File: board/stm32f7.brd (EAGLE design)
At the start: 38 x 37.7 mm, 34 parts, among them Q1 8MHz, U1 STM32F722XX, X1 MINI-USB-32005-201

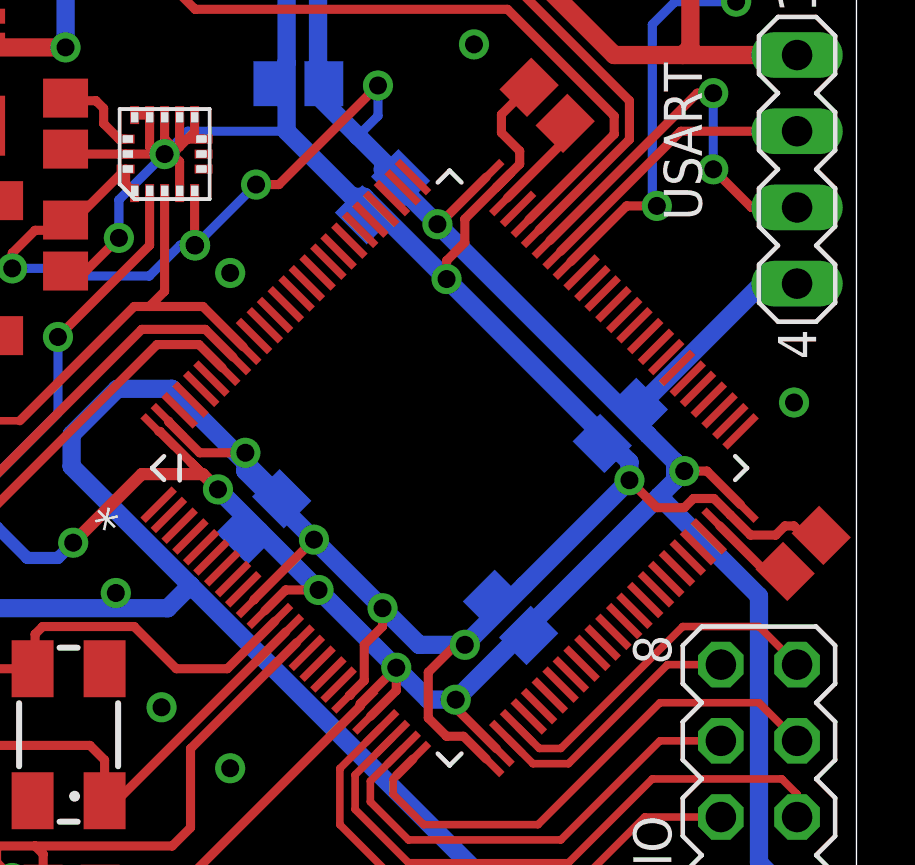
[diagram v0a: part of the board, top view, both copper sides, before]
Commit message: ir cam
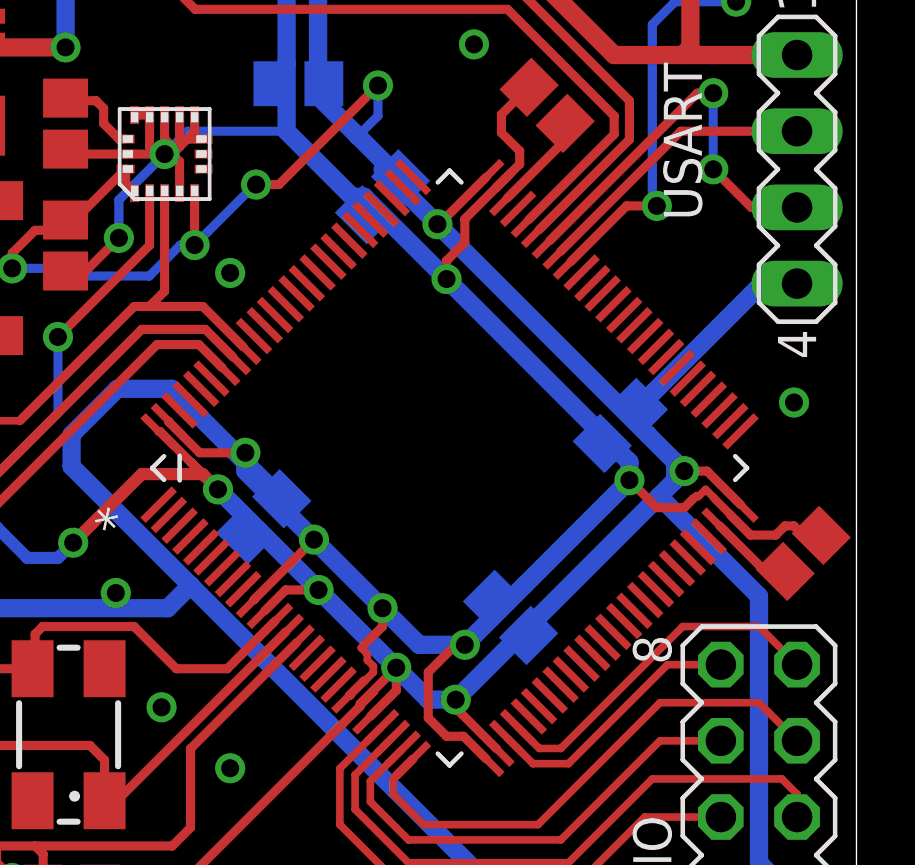
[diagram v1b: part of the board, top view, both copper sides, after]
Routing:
- net GND: track 227.7 -> 228.4 mm
- net +3V3: vias 13 -> 12
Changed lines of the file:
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@@
 <setting verticaltext="up"/>
 </settings>
-<grid distance="10" unitdist="mil" unit="mil" style="lines" multiple="1" display="no" altdistance="0.025" altunitdist="inch" altunit="inch"/>
+<grid distance="8" unitdist="mil" unit="mil" style="lines" multiple="1" display="yes" altdistance="0.025" altunitdist="inch" altunit="inch"/>
 <layers>
 <layer number="1" name="Top" color="4" fill="1" visible="yes" active="yes"/>
@@
 <wire x1="31.3944" y1="14.6304" x2="32.3088" y2="14.6304" width="0.3048" layer="1"/>
 <wire x1="32.3088" y1="14.6304" x2="32.6136" y2="14.9352" width="0.3048" layer="1"/>
-<wire x1="33.296459375" y1="14.9352" x2="33.843025" y2="14.388634375" width="0.3048" layer="1"/>
 <wire x1="23.4696" y1="10.0584" x2="22.2504" y2="11.2776" width="0.3048" layer="16"/>
 <via x="22.2504" y="11.2776" extent="1-16" drill="0.6"/>
@@
 <wire x1="22.2504" y1="11.2776" x2="22.2504" y2="10.668" width="0.3048" layer="1"/>
 <wire x1="22.2504" y1="10.668" x2="21.6408" y2="10.0584" width="0.3048" layer="1"/>
-<wire x1="21.6408" y1="10.0584" x2="21.6408" y2="8.86771875" width="0.3048" layer="1"/>
 <wire x1="21.6408" y1="8.86771875" x2="21.14494375" y2="8.3718625" width="0.3048" layer="1"/>
 <wire x1="30.48" y1="15.5448" x2="30.48" y2="16.1544" width="0.6096" layer="16"/>
@@
 <contactref element="C16" pad="2"/>
 <contactref element="LED2" pad="C"/>
-<wire x1="32.6136" y1="14.9352" x2="33.296459375" y2="14.9352" width="0.3048" layer="1"/>
 <wire x1="7.9248" y1="11.2776" x2="7.6962" y2="11.5062" width="0.6096" layer="16"/>
 <via x="6.4008" y="12.8016" extent="1-16" drill="0.6"/>
@@
 <vertex x="-10.16" y="-18.034"/>
 </polygon>
+<wire x1="21.6408" y1="8.86771875" x2="21.66931875" y2="8.86771875" width="0.254" layer="1"/>
+<wire x1="21.66931875" y1="8.86771875" x2="21.9456" y2="9.144" width="0.254" layer="1"/>
+<wire x1="21.9456" y1="9.144" x2="21.9456" y2="9.3472" width="0.254" layer="1"/>
+<wire x1="21.9456" y1="9.3472" x2="21.7424" y2="9.5504" width="0.254" layer="1"/>
+<wire x1="21.7424" y1="9.5504" x2="21.7424" y2="9.7536" width="0.254" layer="1"/>
+<wire x1="21.7424" y1="9.7536" x2="21.5392" y2="9.9568" width="0.254" layer="1"/>
+<wire x1="21.5392" y1="9.9568" x2="21.6408" y2="10.0584" width="0.254" layer="1"/>
+<wire x1="32.6136" y1="14.9352" x2="32.7152" y2="15.0368" width="0.254" layer="1"/>
+<wire x1="33.843025" y1="14.388634375" x2="33.843025" y2="14.416975" width="0.254" layer="1"/>
+<wire x1="33.843025" y1="14.416975" x2="33.274" y2="14.986" width="0.254" layer="1"/>
+<wire x1="33.296459375" y1="14.9352" x2="33.296459375" y2="14.963540625" width="0.254" layer="1"/>
+<wire x1="33.296459375" y1="14.963540625" x2="33.02" y2="15.24" width="0.254" layer="1"/>
+<wire x1="33.02" y1="15.24" x2="32.766" y2="14.986" width="0.254" layer="1"/>
 </signal>
 <signal name="RESET">
@@
 <wire x1="11.988" y1="24.218" x2="13.686" y2="25.916" width="0.3048" layer="1"/>
 <wire x1="15.986" y1="25.116" x2="15.986" y2="23.384" width="0.3048" layer="1"/>
-<wire x1="15.986" y1="23.384" x2="16.002" y2="23.368" width="0.3048" layer="1"/>
-<via x="16.002" y="23.368" extent="1-16" drill="0.6"/>
 <wire x1="15.51" y1="23.384" x2="14.478" y2="22.352" width="0.3048" layer="16"/>
 <wire x1="14.478" y1="22.352" x2="11.684" y2="22.352" width="0.3048" layer="16"/>
@@
 <wire x1="10.668" y1="23.876" x2="11.342" y2="23.876" width="0.3048" layer="1"/>
 <wire x1="11.342" y1="23.876" x2="11.684" y2="24.218" width="0.3048" layer="1"/>
-<wire x1="16.002" y1="23.368" x2="18.034" y2="25.4" width="0.3048" layer="16"/>
 <via x="18.034" y="25.4" extent="1-16" drill="0.6"/>
 <wire x1="18.034" y1="25.4" x2="18.796" y2="25.4" width="0.3048" layer="1"/>
@@
 <via x="15.986" y="23.384" extent="1-16" drill="0.6"/>
 <wire x1="15.986" y1="23.384" x2="15.51" y2="23.384" width="0.3048" layer="16"/>
+<wire x1="18.034" y1="25.4" x2="18.002" y2="25.4" width="0.3048" layer="16"/>
+<wire x1="18.002" y1="25.4" x2="15.986" y2="23.384" width="0.3048" layer="16"/>
 </signal>
 <signal name="BOOT">
